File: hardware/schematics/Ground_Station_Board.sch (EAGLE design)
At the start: 11 parts

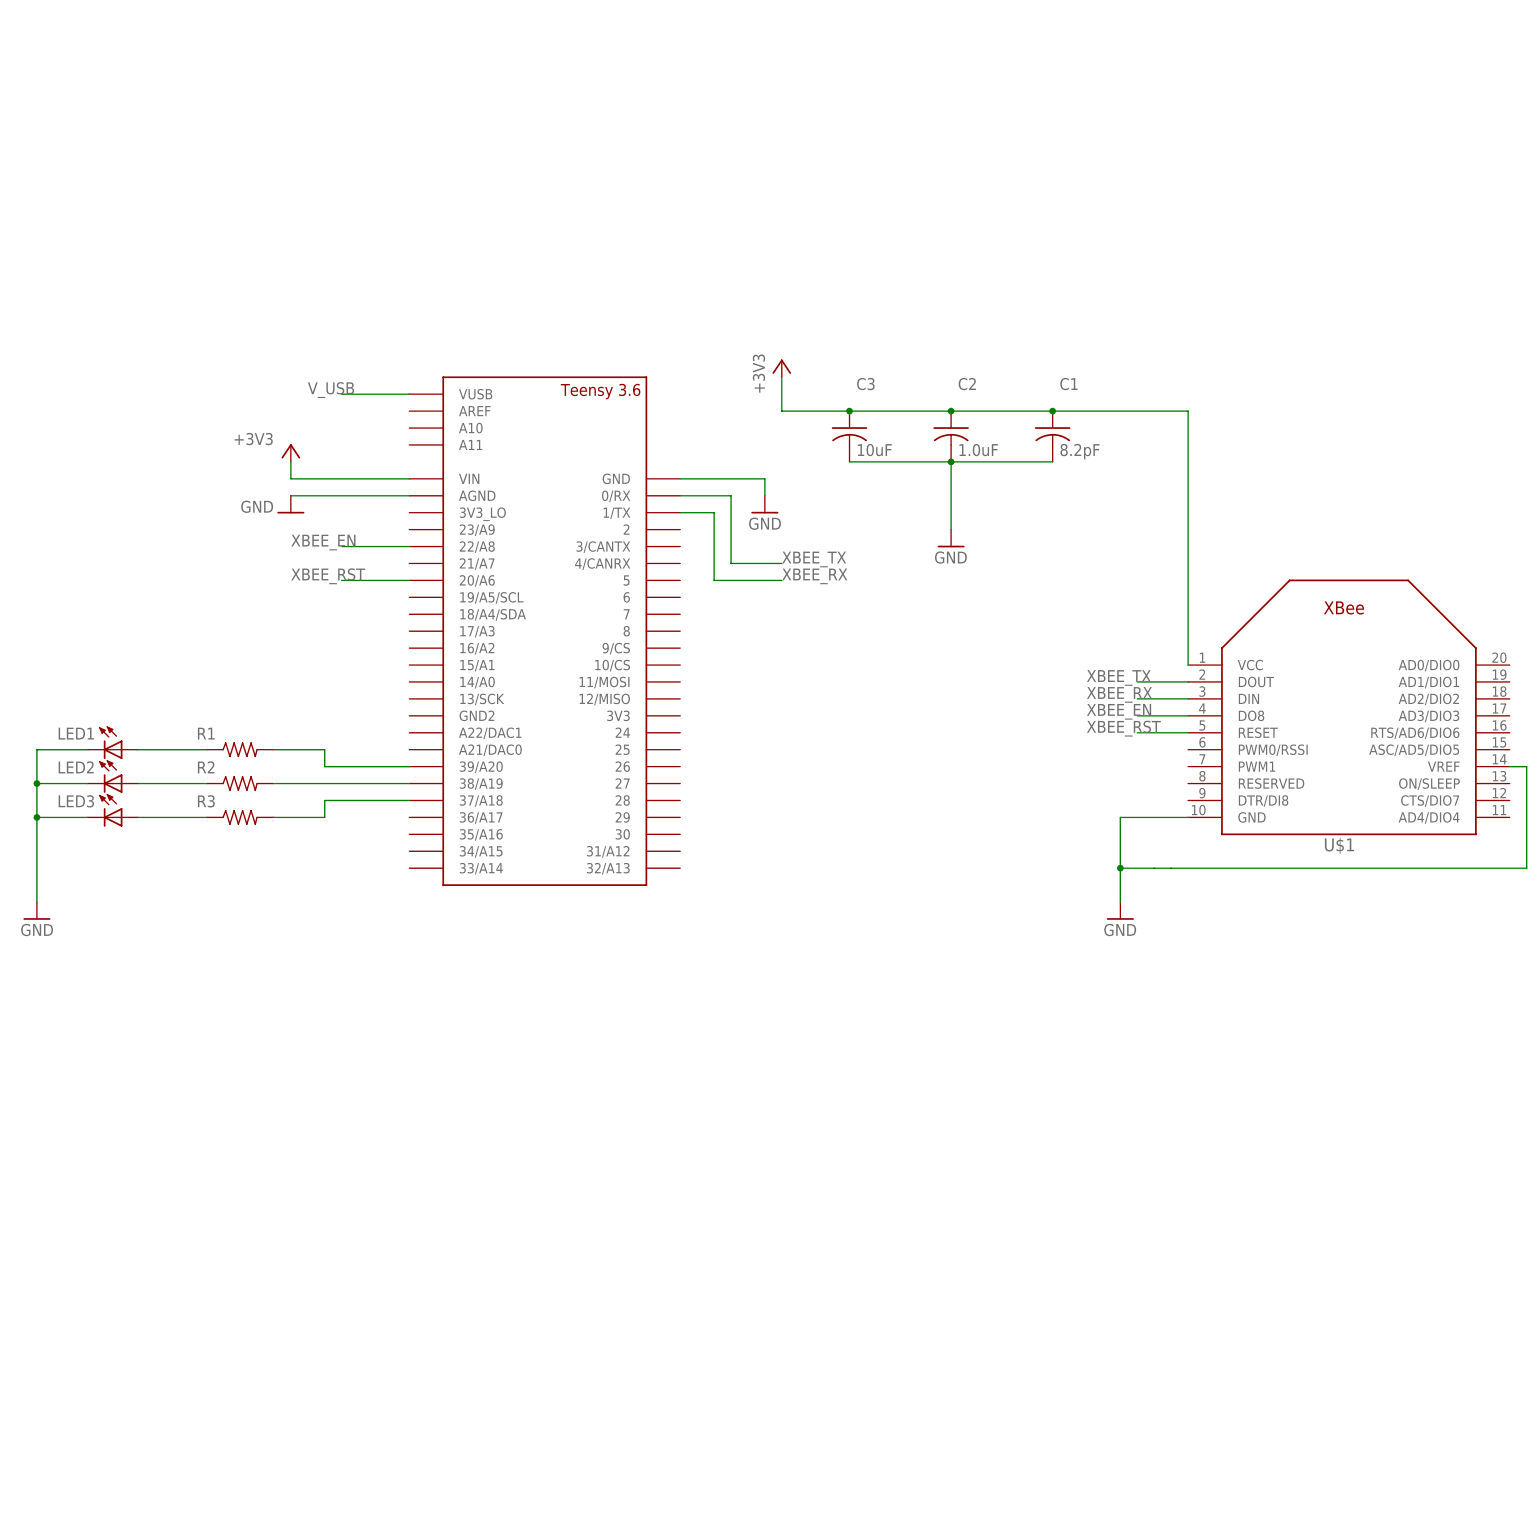
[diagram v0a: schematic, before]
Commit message: Add files via upload
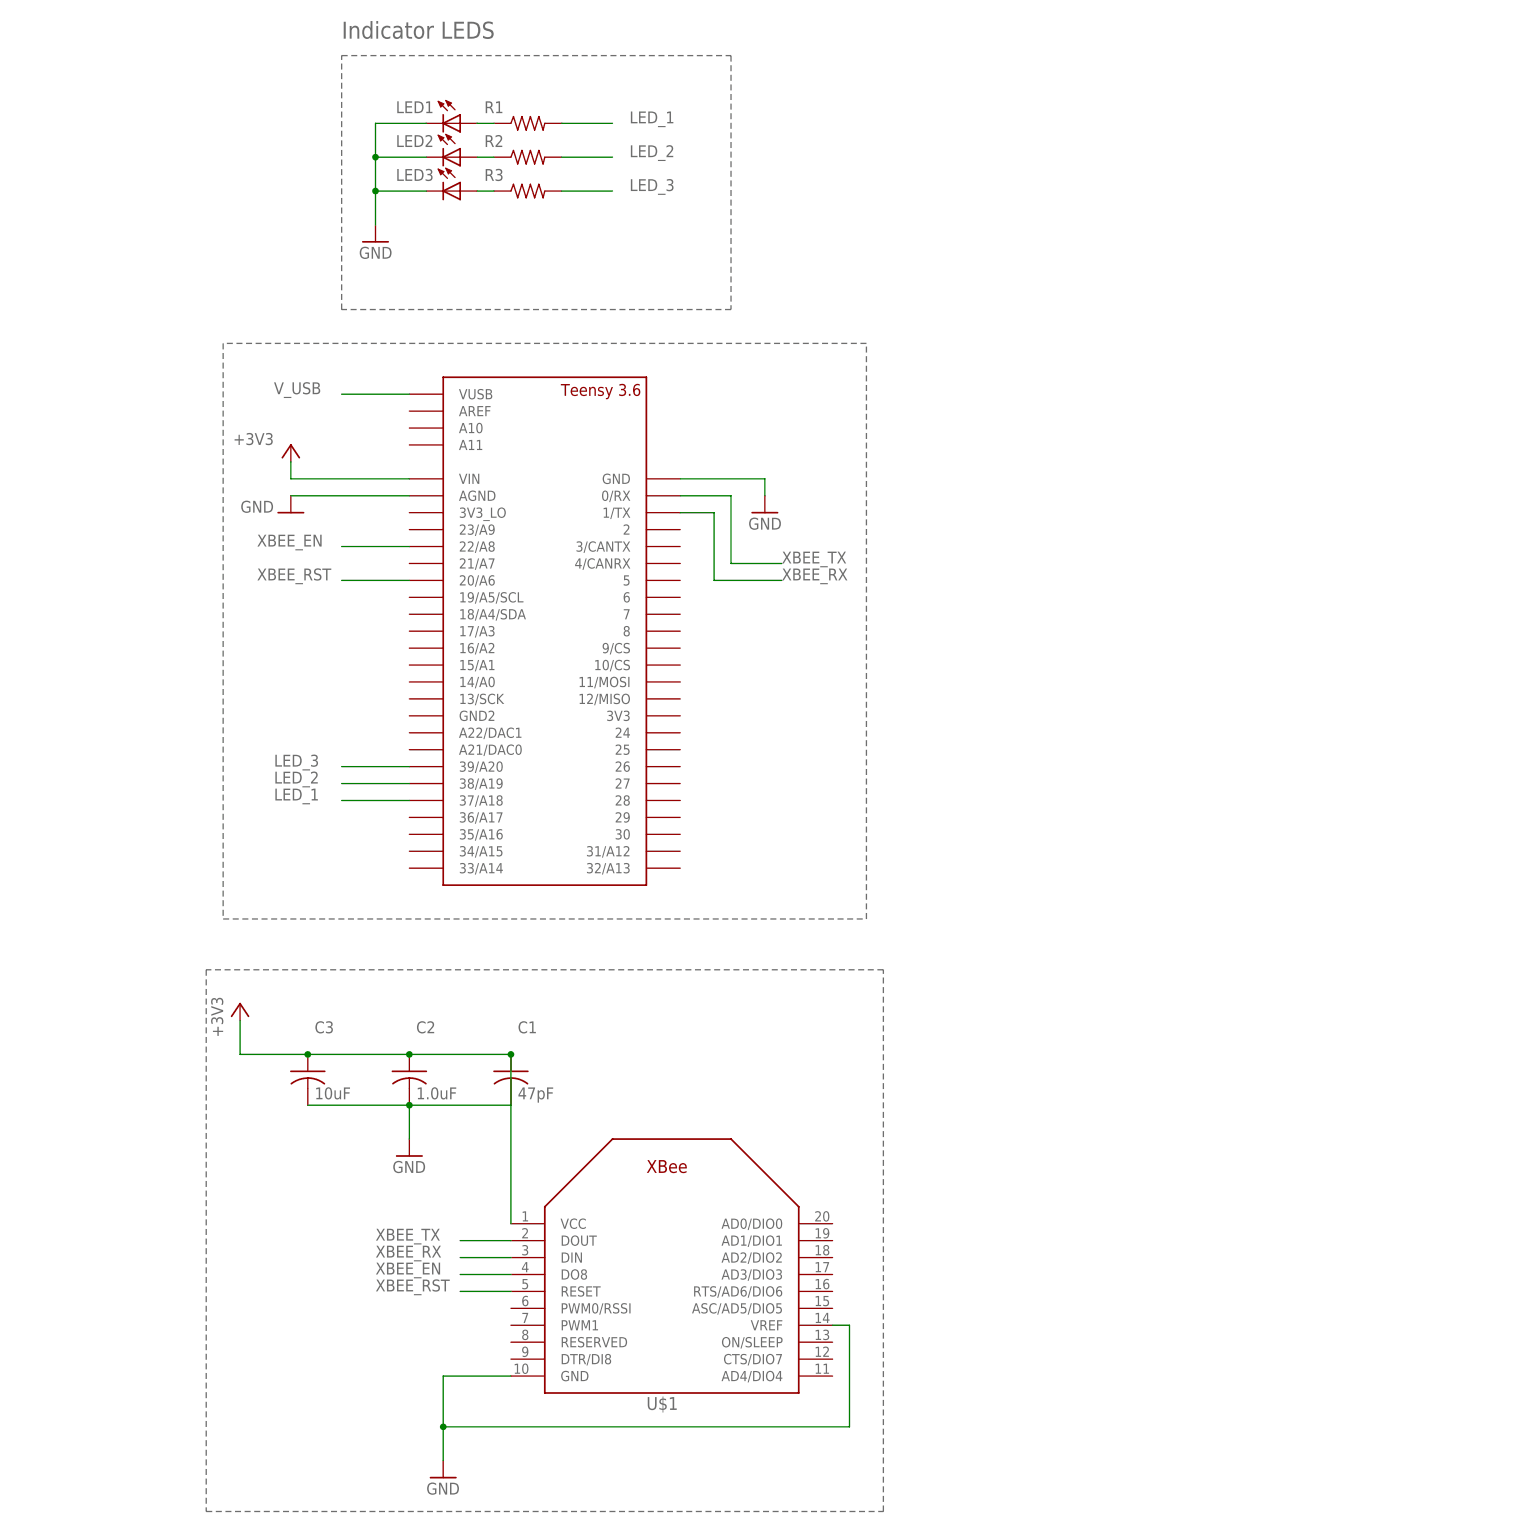
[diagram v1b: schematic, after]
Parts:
- C1: value 8.2pF -> 47pF
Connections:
- net N$2 renamed LED_2
- removed net N$1: R3.2, U$2.37/A18
- removed net N$3: R1.2, U$2.39/A20
- new net LED_1: R1.2, U$2.37/A18
- new net LED_3: R3.2, U$2.39/A20
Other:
- note added: "Indicator LEDS"
- moved on the sheet: C1, C2, C3, LED1, LED2, LED3, R1, R2, R3, U$1
